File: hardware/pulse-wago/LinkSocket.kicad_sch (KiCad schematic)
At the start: 4 parts, among them J2001 2x05_Horizontal, U2001 THVD24x2

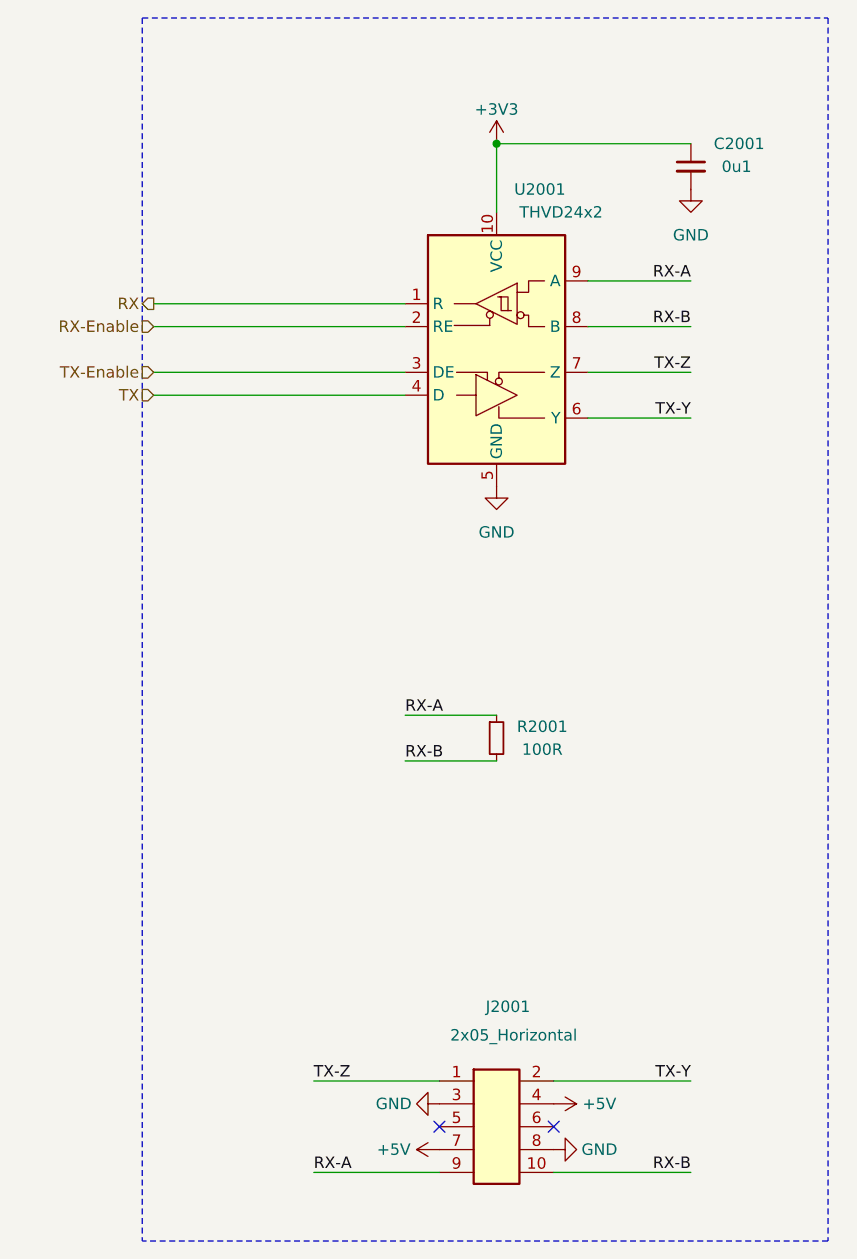
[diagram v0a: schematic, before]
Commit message: Update library
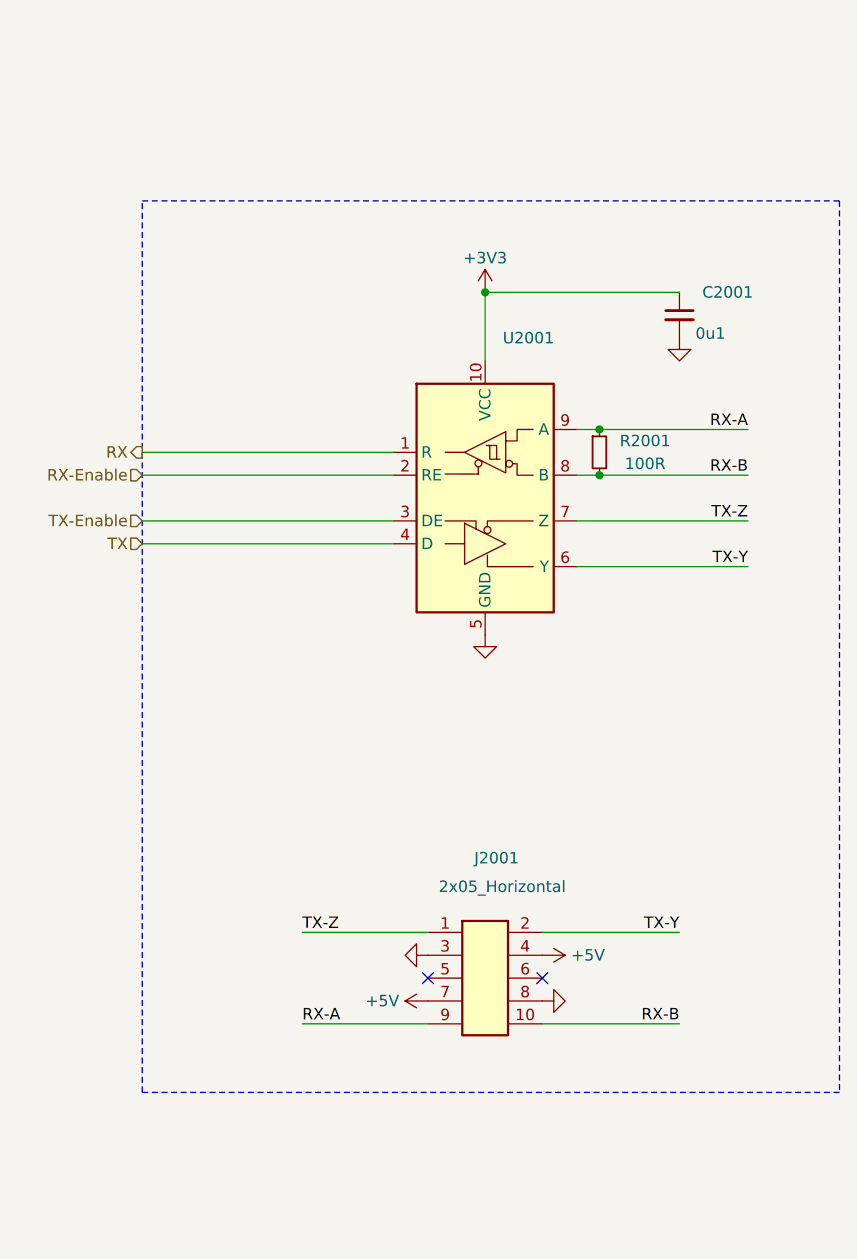
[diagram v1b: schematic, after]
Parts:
- C2001: footprint Capacitor_SMD:C_0603_1608Metric -> V2_Capacitor_SMD:C_0603; symbol Device:C_Small -> V2_Device:C_0603_0u1; Manufacturer (none) -> TDK; Mouser (none) -> 810-CGA3E2X7R1H104MA; Product (none) -> CGA3E2X7R1H104M080AA; Rating (none) -> 50V
- J2001: Manufacturer (none) -> Amphenol FCI; Mouser (none) -> 649-200211120001T4LF; Product (none) -> 20021112-00010T4LF
- R2001: footprint Resistor_SMD:R_0603_1608Metric -> V2_Resistor_SMD:R_0603; symbol Device:R_Small -> V2_Device:R_0603_100R; Manufacturer (none) -> Vishay; Mouser (none) -> 71-CRCW0603100RFKEAH; Product (none) -> CRCW0603100RFKEAHP; Rating (none) -> 330mW
- U2001: value THVD24x2 -> (none)
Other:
- moved on the sheet: C2001, J2001, R2001, U2001

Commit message: Update Library
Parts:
- C2001: symbol V2_Device:C_0603_0u1 -> V2_Capacitor:0603_0u1
- R2001: symbol V2_Device:R_0603_100R -> V2_Resistor:0603_100R
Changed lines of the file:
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@@
 		(on_board yes)
 		(dnp no)
-		(property "Reference" "#PWR02001"
+		(property "Reference" "#PWR2001"
 			(at 151.13 69.85 0)
 			(effects
@@
 			(project "pulse"
 				(path "/6c8448b4-b04d-47e1-934e-e40cbe27a7be/2a03ea79-269e-4abf-833c-000ba0ff13d7"
-					(reference "#PWR02001")
+					(reference "#PWR2001")
 					(unit 1)
 				)
@@
 		(on_board yes)
 		(dnp no)
-		(property "Reference" "#PWR02004"
+		(property "Reference" "#PWR2004"
 			(at 138.43 139.7 0)
 			(effects
@@
 			(project "pulse"
 				(path "/6c8448b4-b04d-47e1-934e-e40cbe27a7be/2a03ea79-269e-4abf-833c-000ba0ff13d7"
-					(reference "#PWR02004")
+					(reference "#PWR2004")
 					(unit 1)
 				)
@@
 		(on_board yes)
 		(dnp no)
-		(property "Reference" "#PWR02003"
+		(property "Reference" "#PWR2003"
 			(at 151.13 110.49 0)
 			(effects
@@
 			(project "pulse"
 				(path "/6c8448b4-b04d-47e1-934e-e40cbe27a7be/2a03ea79-269e-4abf-833c-000ba0ff13d7"
-					(reference "#PWR02003")
+					(reference "#PWR2003")
 					(unit 1)
 				)
@@
 		(on_board yes)
 		(dnp no)
-		(property "Reference" "#PWR02002"
+		(property "Reference" "#PWR2002"
 			(at 172.72 77.47 0)
 			(effects
@@
 			(project "pulse"
 				(path "/6c8448b4-b04d-47e1-934e-e40cbe27a7be/2a03ea79-269e-4abf-833c-000ba0ff13d7"
-					(reference "#PWR02002")
-					(unit 1)
-				)
-			)
-		)
-	)
-	(symbol
-		(lib_id "V2_Device:R_0603_100R")
+					(reference "#PWR2002")
+					(unit 1)
+				)
+			)
+		)
+	)
+	(symbol
+		(lib_id "V2_Resistor:0603_100R")
 		(at 163.83 83.82 0)
 		(unit 1)
@@
 		(on_board yes)
 		(dnp no)
-		(property "Reference" "#PWR02007"
+		(property "Reference" "#PWR2007"
 			(at 163.83 144.78 0)
 			(effects
@@
 			(project "pulse"
 				(path "/6c8448b4-b04d-47e1-934e-e40cbe27a7be/2a03ea79-269e-4abf-833c-000ba0ff13d7"
-					(reference "#PWR02007")
+					(reference "#PWR2007")
 					(unit 1)
 				)
@@
 	)
 	(symbol
-		(lib_id "V2_Device:C_0603_0u1")
+		(lib_id "V2_Capacitor:0603_0u1")
 		(at 172.72 68.58 0)
 		(unit 1)
@@
 		(on_board yes)
 		(dnp no)
-		(property "Reference" "#PWR02006"
+		(property "Reference" "#PWR2006"
 			(at 148.59 144.78 0)
 			(effects
@@
 			(project "pulse"
 				(path "/6c8448b4-b04d-47e1-934e-e40cbe27a7be/2a03ea79-269e-4abf-833c-000ba0ff13d7"
-					(reference "#PWR02006")
+					(reference "#PWR2006")
 					(unit 1)
 				)
@@
 		(on_board yes)
 		(dnp no)
-		(property "Reference" "#PWR02005"
+		(property "Reference" "#PWR2005"
 			(at 153.67 139.7 0)
 			(effects
@@
 			(project "pulse"
 				(path "/6c8448b4-b04d-47e1-934e-e40cbe27a7be/2a03ea79-269e-4abf-833c-000ba0ff13d7"
-					(reference "#PWR02005")
-					(unit 1)
-				)
+					(reference "#PWR2005")
+					(unit 1)
+				)

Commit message: Update ESD suppressor
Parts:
- U2001: value (none) -> ~
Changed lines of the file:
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@@
 			)
 		)
-		(property "Value" ""
+		(property "Value" "~"
 			(at 153.67 73.66 0)
 			(effects
